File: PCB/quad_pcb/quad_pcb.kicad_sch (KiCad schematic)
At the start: 113 parts, among them J1 Screw_Terminal_01x02, J10 Screw_Terminal_01x02, J11 Screw_Terminal_01x02, J12 Screw_Terminal_01x02, J13 Screw_Terminal_01x02, J14 Screw_Terminal_01x03, J15 Screw_Terminal_01x03, J16 Screw_Terminal_01x03, J17 Screw_Terminal_01x03, J2 Screw_Terminal_01x02, J3 Screw_Terminal_01x02, J4 Screw_Terminal_01x02, J5 Screw_Terminal_01x02, J6 Screw_Terminal_01x02, J7 Screw_Terminal_01x02, J8 Screw_Terminal_01x02, J9 Screw_Terminal_01x02, U1 ESP32-S3-WROOM-1, U10 DRV8871DDA, U11 DRV8871DDA, U12 DRV8871DDA, U13 DRV8871DDA, U14 DRV8871DDA, U15 DRV8871DDA, U16 PCA9685PW, U17 PCA9685PW, U2 AP63203WU, U3 AMS1117-3.3, U4 DRV8871DDA, U5 DRV8871DDA, U6 DRV8871DDA, U7 DRV8871DDA, U8 DRV8871DDA, U9 DRV8871DDA

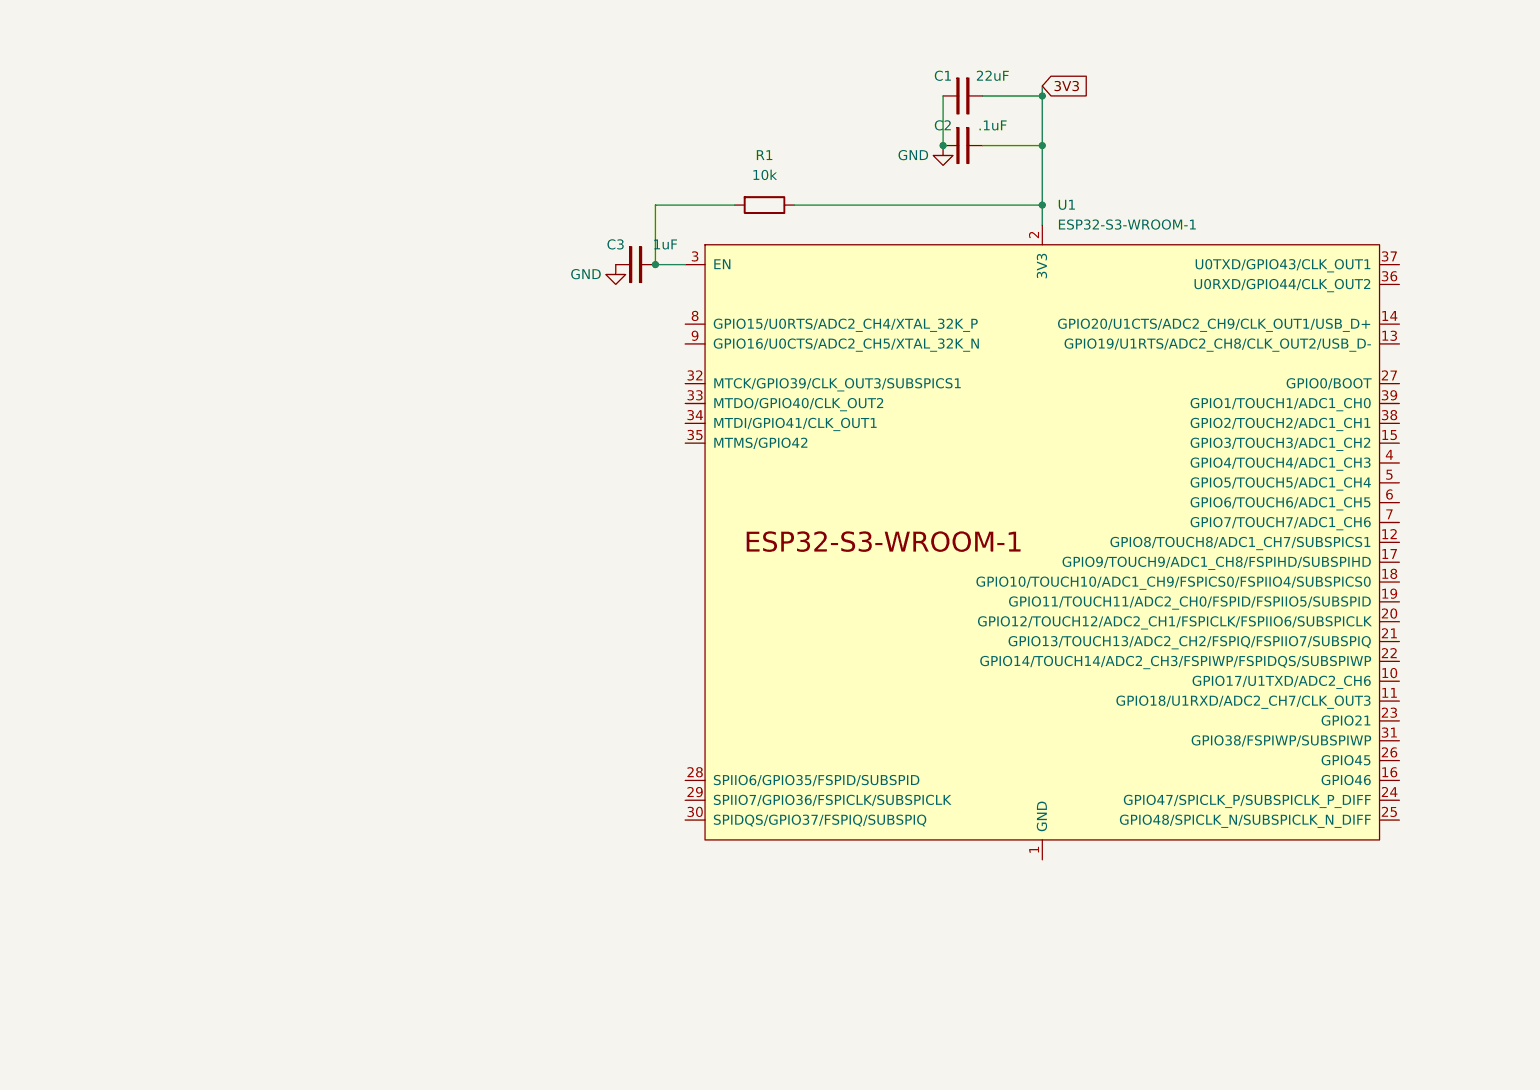
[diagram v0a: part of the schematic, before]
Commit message: small changes
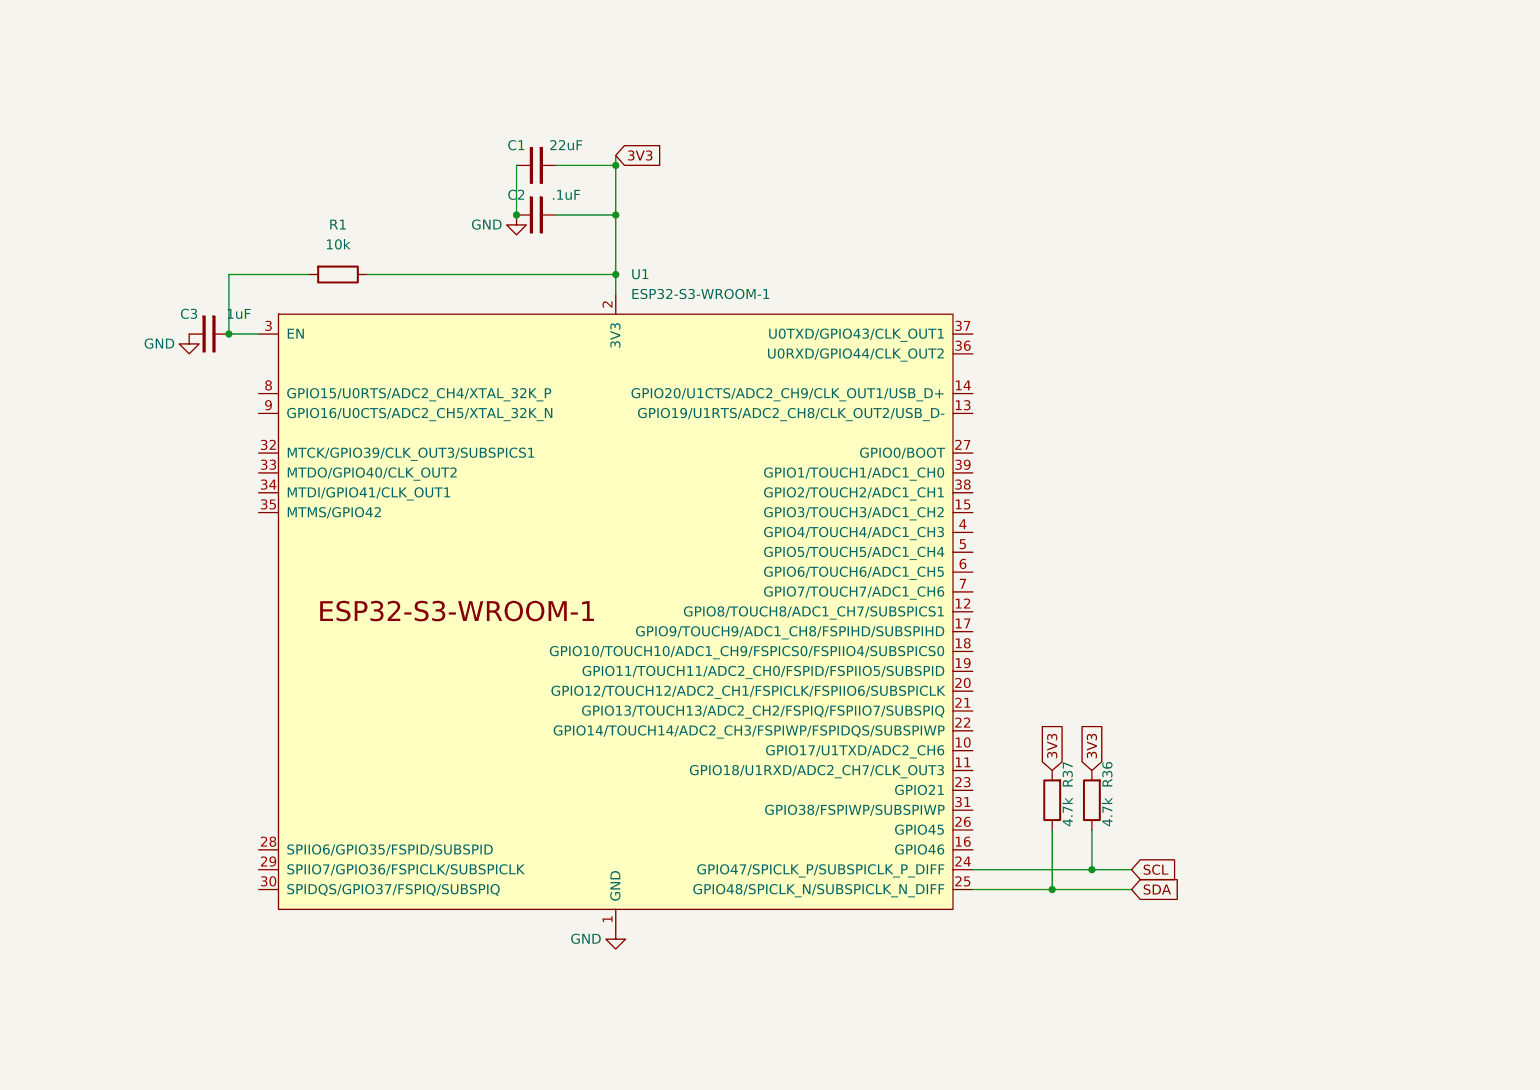
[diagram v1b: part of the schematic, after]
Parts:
- added R36, R37: 4.7k, symbol Device:R
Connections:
- net 3V3: now also R36.2, R37.2
- net GND: now also U1.1 (GND), U1.40 (GND), U1.41 (GND)
- net SCL: now also U1.24 (GPIO47/SPICLK_P/SUBSPICLK_P_DIFF), R36.1
- net SDA: now also U1.25 (GPIO48/SPICLK_N/SUBSPICLK_N_DIFF), R37.1
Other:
- moved on the sheet: C1, C2, C3, R1, U1
